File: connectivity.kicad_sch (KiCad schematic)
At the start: 28 parts, among them J10 Screw_Terminal_01x05, J11 RJ45_Hanrun_HR911105A_Horizon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, J8 Conn_02x01, J9 Conn_02x01, U10 LAN8742A, U9 TJA1042T-3, Y3 25 MHz

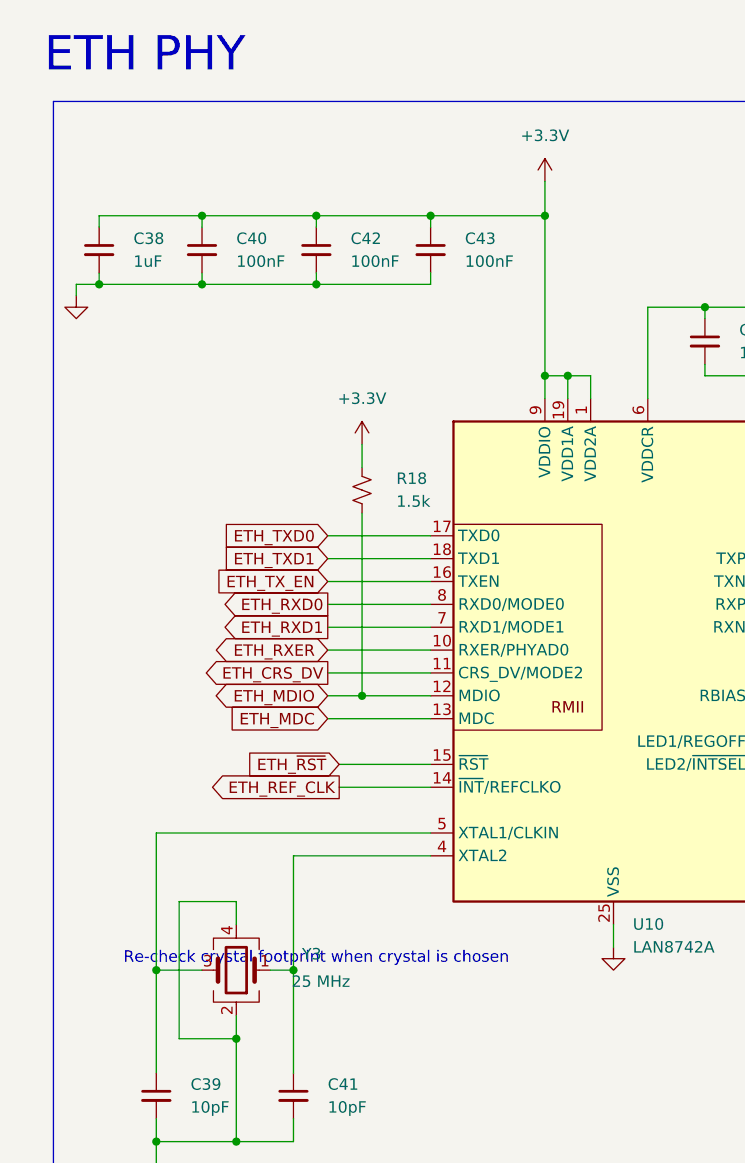
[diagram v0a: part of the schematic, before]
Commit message: Initial release A1
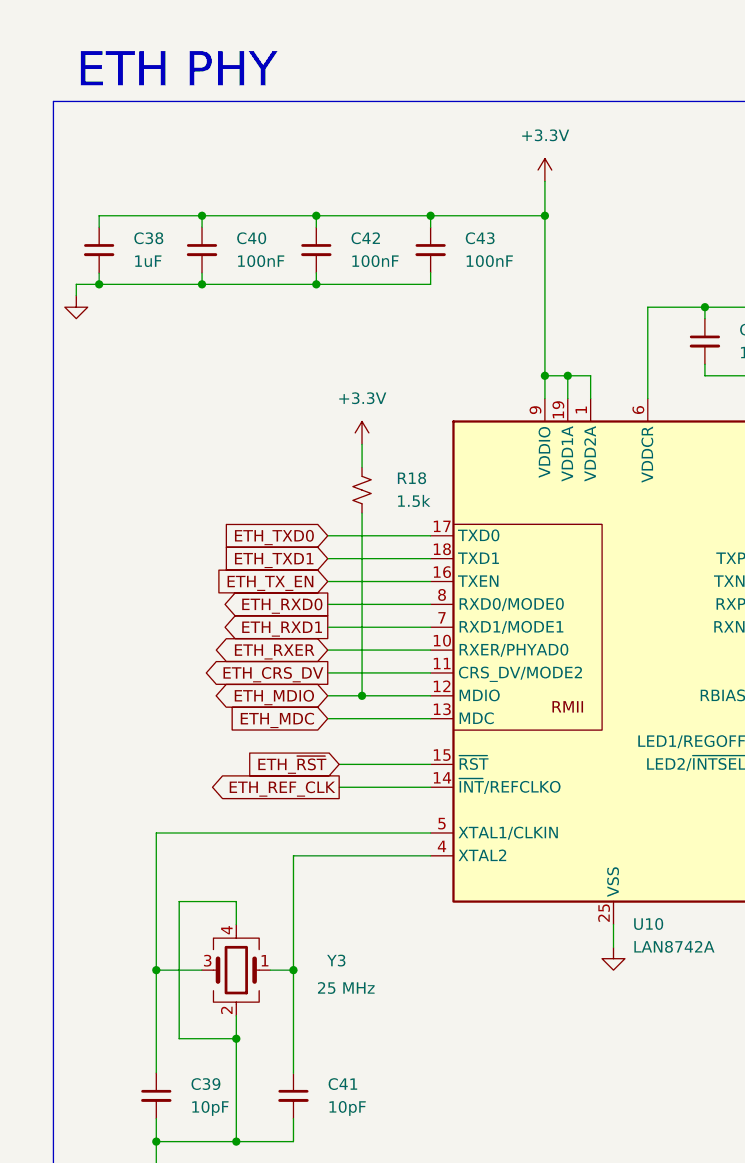
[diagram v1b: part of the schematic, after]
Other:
- note removed: "Re-check crystal footprint when crystal is chosen"
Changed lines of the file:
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@@
 	(title_block
 		(title "PT DAQ")
-		(date "2026-01-01")
+		(date "2026-01-12")
 		(rev "1A")
 		(company "Aggie Propulsion and Rocketry Lab")
@@
 	(text "ETH PHY"
 		(exclude_from_sim no)
-		(at 26.67 19.05 0)
+		(at 30.226 20.828 0)
 		(effects
 			(font
@@
 		)
 	)
-	(text "Re-check crystal footprint when crystal is chosen"
-		(exclude_from_sim no)
-		(at 45.72 119.38 0)
-		(effects
-			(font
-				(size 1.27 1.27)
-			)
-		)
-	)
 	(text "CAN"
 		(exclude_from_sim no)
@@
 		(dnp no)
 		(property "Reference" "Y3"
-			(at 45.212 118.872 0)
+			(at 48.006 119.634 0)
 			(effects
 				(font
@@
 		)
 		(property "Value" "25 MHz"
-			(at 46.228 121.92 0)
+			(at 49.022 122.682 0)
 			(effects
 				(font
